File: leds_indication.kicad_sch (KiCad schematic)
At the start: 8 parts, among them U8 74HC595

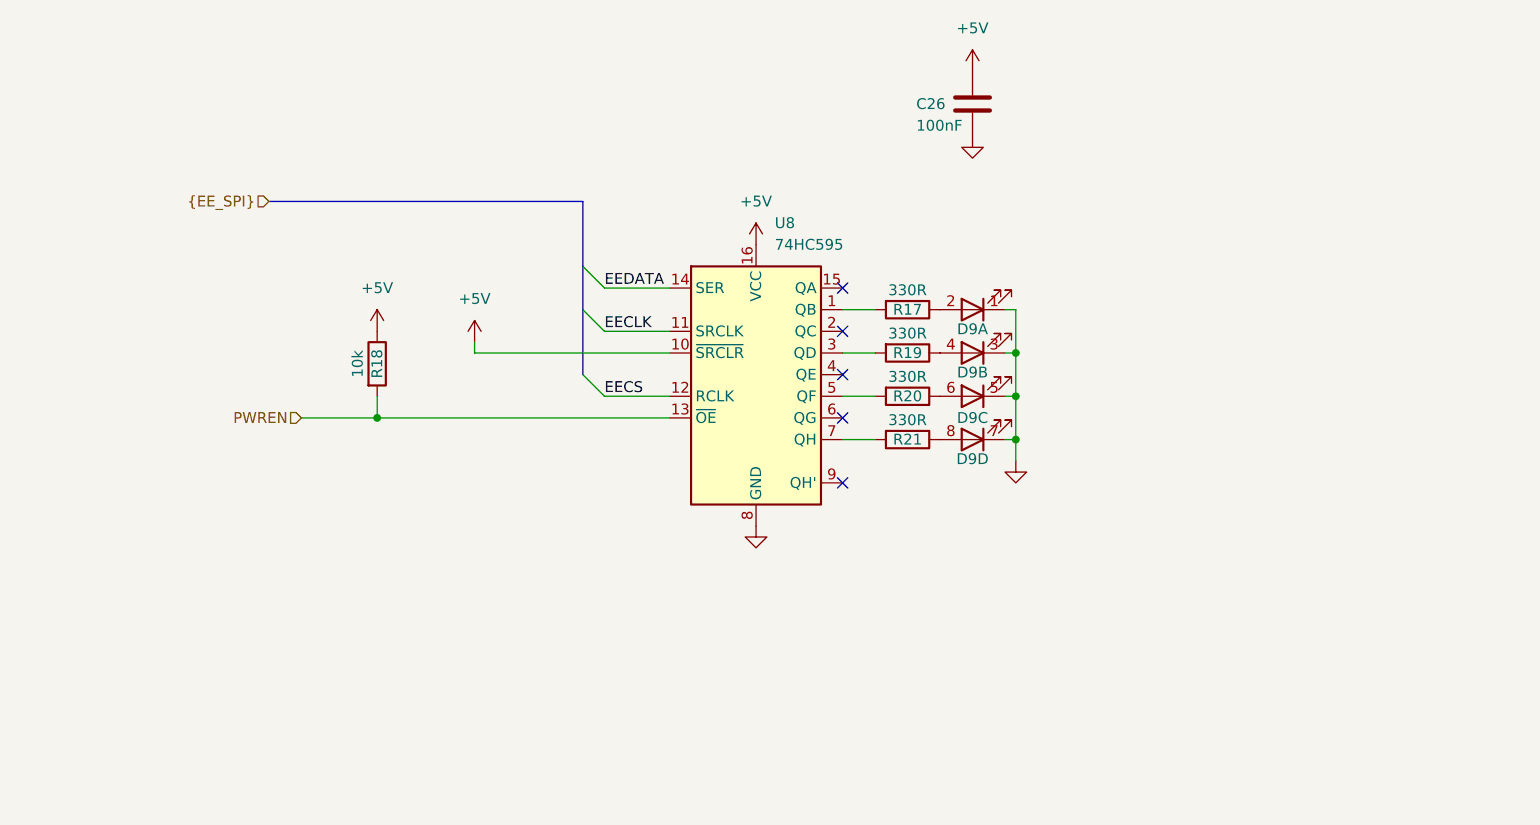
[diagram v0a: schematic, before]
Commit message: progress
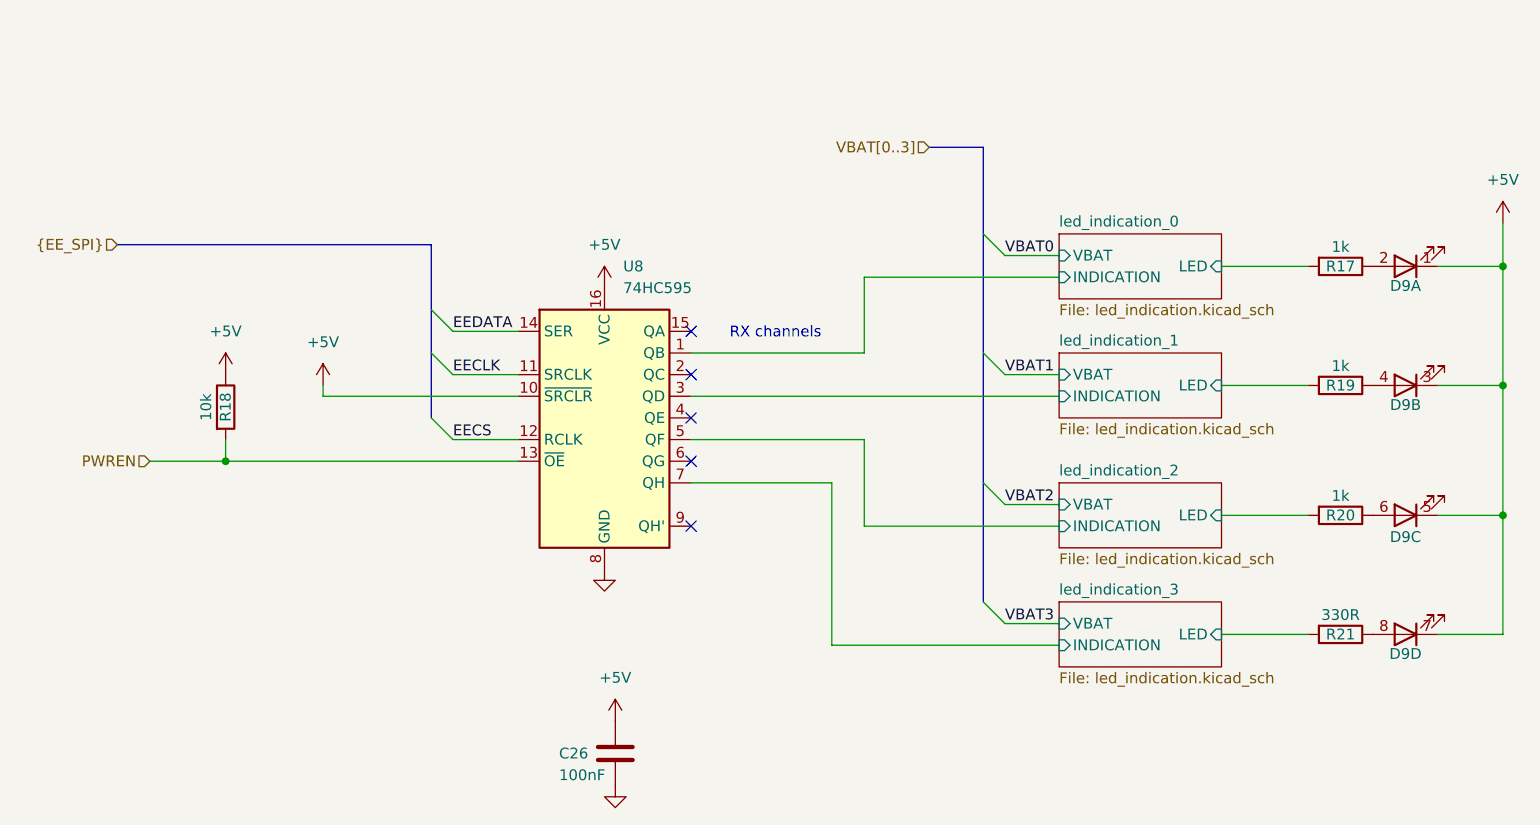
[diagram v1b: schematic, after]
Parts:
- D9: footprint ftdi_quad_lin:1296.3004 -> ftdi_quad_lin:1276.2004
- R17, R19, R20: value 330R -> 1k
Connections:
- net +5V: now also D9.1, D9.3, D9.5, D9.7
- net GND: no longer D9.1, D9.3, D9.5, D9.7
- net led_indication_2/INDICATION: now reaches U8.5 (QF)
- net led_indication_2/INDICATION: no longer R20.2
- net led_indication_1/INDICATION: now reaches U8.3 (QD)
- net led_indication_1/INDICATION: no longer R19.2
- net led_indication_3/INDICATION: now reaches U8.7 (QH)
- net led_indication_3/INDICATION: no longer R21.2
- net led_indication_0/INDICATION: now reaches U8.1 (QB)
- net led_indication_0/INDICATION: no longer R17.2
- new net led_indication_0/LED: R17.2
- new net led_indication_1/LED: R19.2
- new net led_indication_2/LED: R20.2
- new net led_indication_3/LED: R21.2
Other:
- added sheet led_indication_0 (led_indication.kicad_sch)
- added sheet led_indication_1 (led_indication.kicad_sch)
- added sheet led_indication_2 (led_indication.kicad_sch)
- added sheet led_indication_3 (led_indication.kicad_sch)
- note added: "RX channels"
- moved on the sheet: C26, D9A, D9B, D9C, D9D, R17, R18, R19, R20, R21, U8
